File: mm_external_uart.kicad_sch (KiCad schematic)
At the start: 0 parts

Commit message: fin tp2
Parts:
- added C7, C8: 10uf, symbol Device:C
- added J4: Conn_01x04_Pin, Connector_PinHeader_2.54mm:PinHeader_1x04_P2.54mm_Vertical, symbol Connector:Conn_01x04_Pin
- added RTX: 100, symbol Device:R
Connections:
- new net: J4.4 (Pin_4), RTX.1
- new net +BATT: C8.2, J4.1 (Pin_1)
- new net EXT_UART_RX: RTX.2
- new net EXT_UART_TX: C7.2, J4.3 (Pin_3)
- new net GND: C7.1, C8.1, J4.2 (Pin_2)

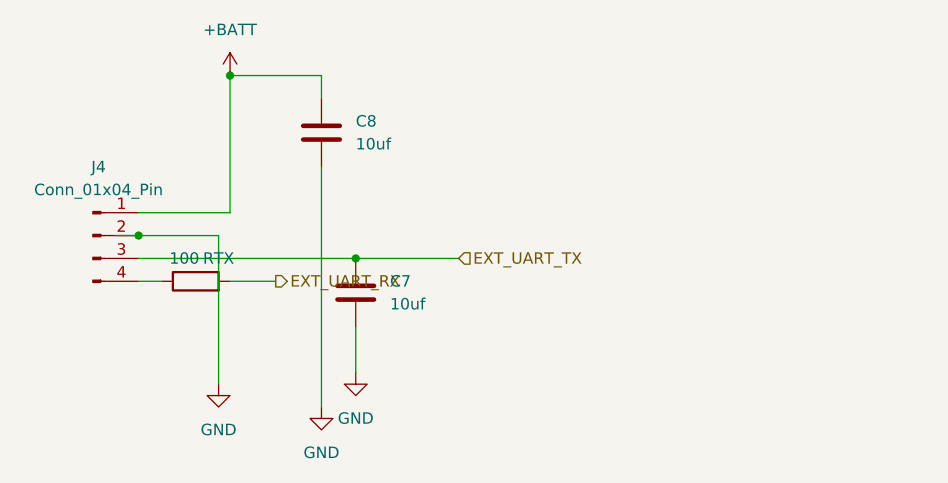
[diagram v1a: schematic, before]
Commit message: TP3
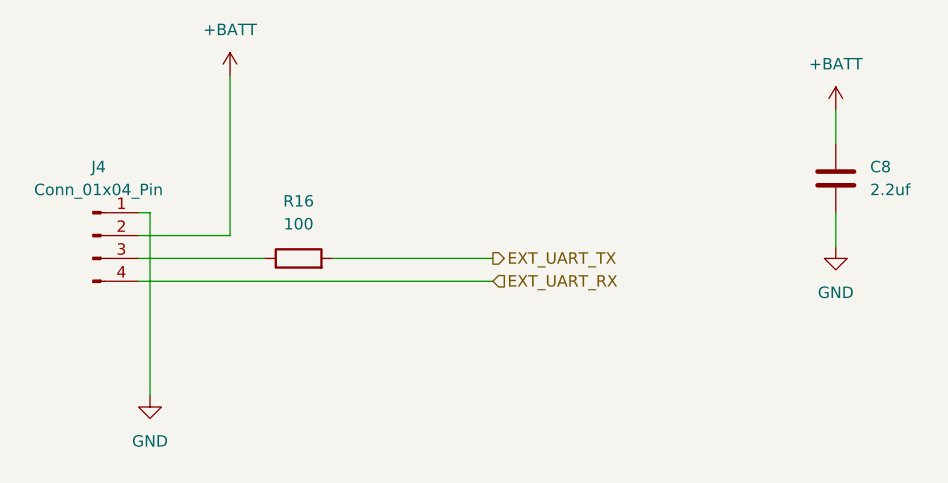
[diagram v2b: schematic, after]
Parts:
- removed C7: 10uf, symbol Device:C
- removed RTX: 100, symbol Device:R
- added R16: 100, Resistor_SMD:R_0603_1608Metric, symbol Device:R
- C8: value 10uf -> 2.2uf; footprint (none) -> Capacitor_SMD:C_0603_1608Metric
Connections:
- net +BATT: now also J4.2 (Pin_2); no longer J4.1 (Pin_1)
- net EXT_UART_RX: now also J4.4 (Pin_4)
- net EXT_UART_TX: now also R16.2; no longer J4.3 (Pin_3)
- net GND: now also J4.1 (Pin_1); no longer J4.2 (Pin_2)
- new net: J4.3 (Pin_3), R16.1
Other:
- moved on the sheet: C8
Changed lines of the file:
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@@
 (kicad_sch (version 20230121) (generator eeschema)
   (paper "A4")
-  (junction (at 162.56 111.76) (diameter 0) (color 0 0 0 0)
-  )
-  (junction (at 172.72 93.98) (diameter 0) (color 0 0 0 0)
-  )
-  (junction (at 186.69 114.3) (diameter 0) (color 0 0 0 0)
-  )
-  (wire (pts (xy 182.88 93.98) (xy 172.72 93.98))
+  (wire (pts (xy 162.56 116.84) (xy 201.93 116.84))
     (stroke (width 0) (type default))
   )
-  (wire (pts (xy 162.56 111.76) (xy 171.45 111.76))
+  (wire (pts (xy 240.03 109.22) (xy 240.03 113.03))
     (stroke (width 0) (type default))
   )
-  (wire (pts (xy 172.72 116.84) (xy 177.8 116.84))
+  (wire (pts (xy 162.56 109.22) (xy 163.83 109.22))
     (stroke (width 0) (type default))
   )
-  (wire (pts (xy 182.88 104.14) (xy 182.88 130.81))
+  (wire (pts (xy 162.56 114.3) (xy 176.53 114.3))
     (stroke (width 0) (type default))
   )
-  (wire (pts (xy 162.56 116.84) (xy 165.1 116.84))
+  (wire (pts (xy 240.03 97.79) (xy 240.03 101.6))
     (stroke (width 0) (type default))
   )
-  (wire (pts (xy 162.56 109.22) (xy 172.72 109.22))
+  (wire (pts (xy 162.56 111.76) (xy 172.72 111.76))
     (stroke (width 0) (type default))
   )
-  (wire (pts (xy 186.69 114.3) (xy 198.12 114.3))
+  (wire (pts (xy 172.72 93.98) (xy 172.72 111.76))
     (stroke (width 0) (type default))
   )
-  (wire (pts (xy 182.88 93.98) (xy 182.88 96.52))
+  (wire (pts (xy 184.15 114.3) (xy 201.93 114.3))
     (stroke (width 0) (type default))
   )
-  (wire (pts (xy 186.69 121.92) (xy 186.69 127))
+  (wire (pts (xy 163.83 109.22) (xy 163.83 129.54))
     (stroke (width 0) (type default))
   )
-  (wire (pts (xy 171.45 111.76) (xy 171.45 128.27))
-    (stroke (width 0) (type default))
-  )
-  (wire (pts (xy 172.72 93.98) (xy 172.72 109.22))
-    (stroke (width 0) (type default))
-  )
-  (wire (pts (xy 160.02 111.76) (xy 162.56 111.76))
-    (stroke (width 0) (type default))
-  )
-  (wire (pts (xy 162.56 114.3) (xy 186.69 114.3))
-    (stroke (width 0) (type default))
-  )
-  (hierarchical_label "EXT_UART_RX" (shape output) (at 177.8 116.84 0) (fields_autoplaced)
+  (hierarchical_label "EXT_UART_RX" (shape input) (at 201.93 116.84 0) (fields_autoplaced)
     (effects (font (size 1.27 1.27)) (justify left))
   )
-  (hierarchical_label "EXT_UART_TX" (shape input) (at 198.12 114.3 0) (fields_autoplaced)
+  (hierarchical_label "EXT_UART_TX" (shape output) (at 201.93 114.3 0) (fields_autoplaced)
     (effects (font (size 1.27 1.27)) (justify left))
   )
-  (symbol (lib_id "power:GND") (at 182.88 130.81 0) (unit 1)
+  (symbol (lib_id "power:GND") (at 240.03 113.03 0) (unit 1)
     (in_bom yes) (on_board yes) (dnp no) (fields_autoplaced)
-    (property "Reference" "#PWR040" (at 182.88 137.16 0)
+    (property "Reference" "#PWR040" (at 240.03 119.38 0)
       (effects (font (size 1.27 1.27)) hide)
     )
-    (property "Value" "GND" (at 182.88 135.89 0)
+    (property "Value" "GND" (at 240.03 118.11 0)
       (effects (font (size 1.27 1.27)))
     )
-    (property "Footprint" "" (at 182.88 130.81 0)
+    (property "Footprint" "" (at 240.03 113.03 0)
       (effects (font (size 1.27 1.27)) hide)
     )
-    (property "Datasheet" "" (at 182.88 130.81 0)
+    (property "Datasheet" "" (at 240.03 113.03 0)
       (effects (font (size 1.27 1.27)) hide)
     )
@@
     )
   )
-  (symbol (lib_id "Device:R") (at 168.91 116.84 90) (unit 1)
-    (in_bom yes) (on_board yes) (dnp no)
-    (property "Reference" "RTX" (at 171.45 114.3 90)
+  (symbol (lib_id "power:+BATT") (at 240.03 97.79 0) (unit 1)
+    (in_bom yes) (on_board yes) (dnp no) (fields_autoplaced)
+    (property "Reference" "#PWR011" (at 240.03 101.6 0)
+      (effects (font (size 1.27 1.27)) hide)
+    )
+    (property "Value" "+BATT" (at 240.03 92.71 0)
       (effects (font (size 1.27 1.27)))
     )
-    (property "Value" "100" (at 167.64 114.3 90)
-      (effects (font (size 1.27 1.27)))
-    )
-    (property "Footprint" "" (at 168.91 118.618 90)
+    (property "Footprint" "" (at 240.03 97.79 0)
       (effects (font (size 1.27 1.27)) hide)
     )
-    (property "Datasheet" "~" (at 168.91 116.84 0)
+    (property "Datasheet" "" (at 240.03 97.79 0)
       (effects (font (size 1.27 1.27)) hide)
     )
     (pin "1")
-    (pin "2")
     (instances
       (project "minimouse"
         (path "/d8fa4cba-2469-4231-847f-065b6b829f44/d17bb1c7-f68a-465e-9a17-5858ef86fc30"
-          (reference "RTX") (unit 1)
+          (reference "#PWR011") (unit 1)
         )
       )
@@
     )
   )
-  (symbol (lib_id "power:GND") (at 186.69 127 0) (unit 1)
+  (symbol (lib_id "power:GND") (at 163.83 129.54 0) (unit 1)
     (in_bom yes) (on_board yes) (dnp no) (fields_autoplaced)
-    (property "Reference" "#PWR039" (at 186.69 133.35 0)
+    (property "Reference" "#PWR031" (at 163.83 135.89 0)
       (effects (font (size 1.27 1.27)) hide)
     )
-    (property "Value" "GND" (at 186.69 132.08 0)
+    (property "Value" "GND" (at 163.83 134.62 0)
       (effects (font (size 1.27 1.27)))
     )
-    (property "Footprint" "" (at 186.69 127 0)
+    (property "Footprint" "" (at 163.83 129.54 0)
       (effects (font (size 1.27 1.27)) hide)
     )
-    (property "Datasheet" "" (at 186.69 127 0)
-      (effects (font (size 1.27 1.27)) hide)
-    )
-    (pin "1")
-    (instances
-      (project "minimouse"
-        (path "/d8fa4cba-2469-4231-847f-065b6b829f44/d17bb1c7-f68a-465e-9a17-5858ef86fc30"
-          (reference "#PWR039") (unit 1)
-        )
-      )
-    )
-  )
-  (symbol (lib_id "power:GND") (at 171.45 128.27 0) (unit 1)
-    (in_bom yes) (on_board yes) (dnp no) (fields_autoplaced)
-    (property "Reference" "#PWR031" (at 171.45 134.62 0)
-      (effects (font (size 1.27 1.27)) hide)
-    )
-    (property "Value" "GND" (at 171.45 133.35 0)
-      (effects (font (size 1.27 1.27)))
-    )
-    (property "Footprint" "" (at 171.45 128.27 0)
-      (effects (font (size 1.27 1.27)) hide)
-    )
-    (property "Datasheet" "" (at 171.45 128.27 0)
+    (property "Datasheet" "" (at 163.83 129.54 0)
       (effects (font (size 1.27 1.27)) hide)
     )
@@
     )
   )
-  (symbol (lib_id "Device:C") (at 182.88 100.33 180) (unit 1)
+  (symbol (lib_id "Device:C") (at 240.03 105.41 180) (unit 1)
     (in_bom yes) (on_board yes) (dnp no) (fields_autoplaced)
-    (property "Reference" "C8" (at 186.69 99.06 0)
+    (property "Reference" "C8" (at 243.84 104.14 0)
       (effects (font (size 1.27 1.27)) (justify right))
     )
-    (property "Value" "10uf" (at 186.69 101.6 0)
+    (property "Value" "2.2uf" (at 243.84 106.68 0)
       (effects (font (size 1.27 1.27)) (justify right))
     )
-    (property "Footprint" "" (at 181.9148 96.52 0)
+    (property "Footprint" "Capacitor_SMD:C_0603_1608Metric" (at 239.0648 101.6 0)
       (effects (font (size 1.27 1.27)) hide)
     )
-    (property "Datasheet" "~" (at 182.88 100.33 0)
+    (property "Datasheet" "~" (at 240.03 105.41 0)
       (effects (font (size 1.27 1.27)) hide)
     )
@@
     )
   )
-  (symbol (lib_id "Device:C") (at 186.69 118.11 180) (unit 1)
+  (symbol (lib_id "Device:R") (at 180.34 114.3 90) (unit 1)
     (in_bom yes) (on_board yes) (dnp no) (fields_autoplaced)
-    (property "Reference" "C7" (at 190.5 116.84 0)
-      (effects (font (size 1.27 1.27)) (justify right))
+    (property "Reference" "R16" (at 180.34 107.95 90)
+      (effects (font (size 1.27 1.27)))
     )
-    (property "Value" "10uf" (at 190.5 119.38 0)
-      (effects (font (size 1.27 1.27)) (justify right))
+    (property "Value" "100" (at 180.34 110.49 90)
+      (effects (font (size 1.27 1.27)))
     )
-    (property "Footprint" "" (at 185.7248 114.3 0)
+    (property "Footprint" "Resistor_SMD:R_0603_1608Metric" (at 180.34 116.078 90)
       (effects (font (size 1.27 1.27)) hide)
     )
-    (property "Datasheet" "~" (at 186.69 118.11 0)
+    (property "Datasheet" "~" (at 180.34 114.3 0)
       (effects (font (size 1.27 1.27)) hide)
     )
@@
       (project "minimouse"
         (path "/d8fa4cba-2469-4231-847f-065b6b829f44/d17bb1c7-f68a-465e-9a17-5858ef86fc30"
-          (reference "C7") (unit 1)
+          (reference "R16") (unit 1)
         )
       )
